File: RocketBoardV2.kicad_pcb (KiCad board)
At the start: 2 copper layers, 12 parts, among them IC1 W25Q256JVEIQ, J1 10118194-0001LF, J3 Conn_01x03_Pin, U1 SC0914_13_, U2 W25Q16JVUXIQ_TR, U3 BMI270, U4 TPS62420DRCR, Y1 ABM8-272-T3

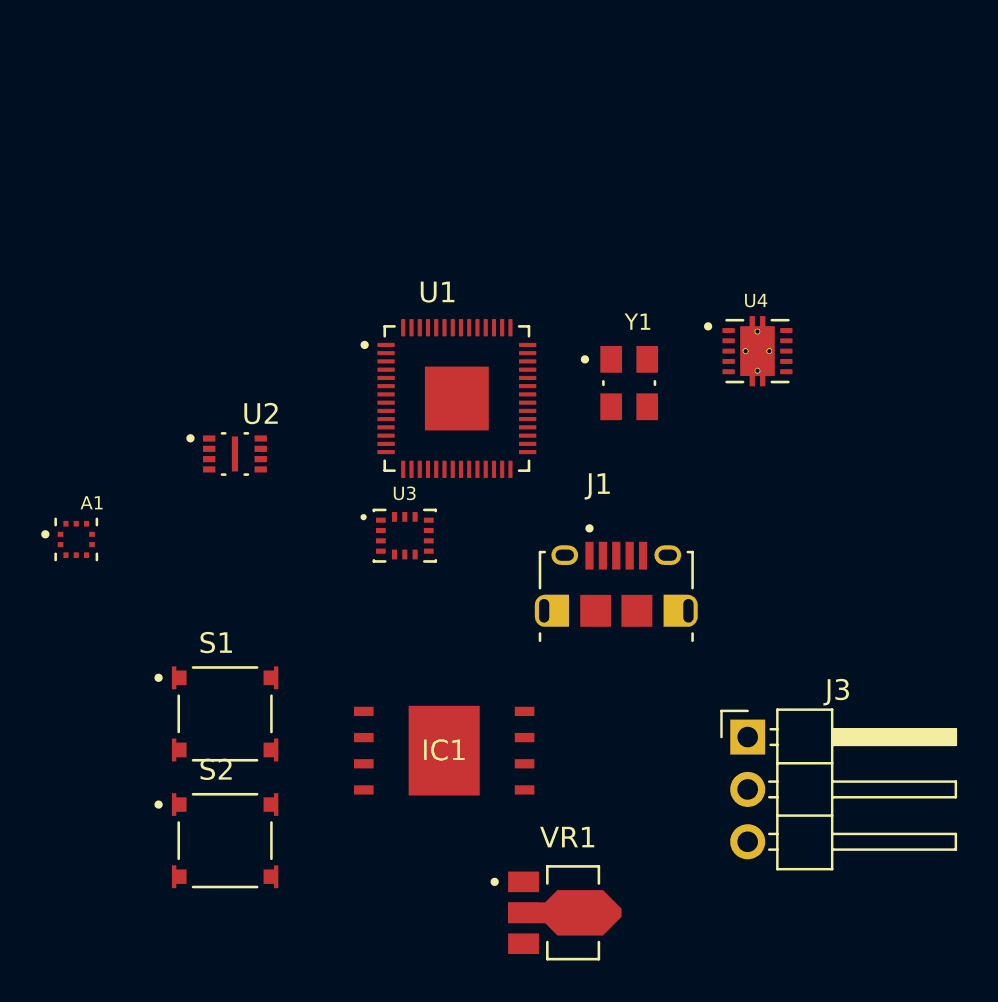
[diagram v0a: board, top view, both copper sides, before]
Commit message: basic layout
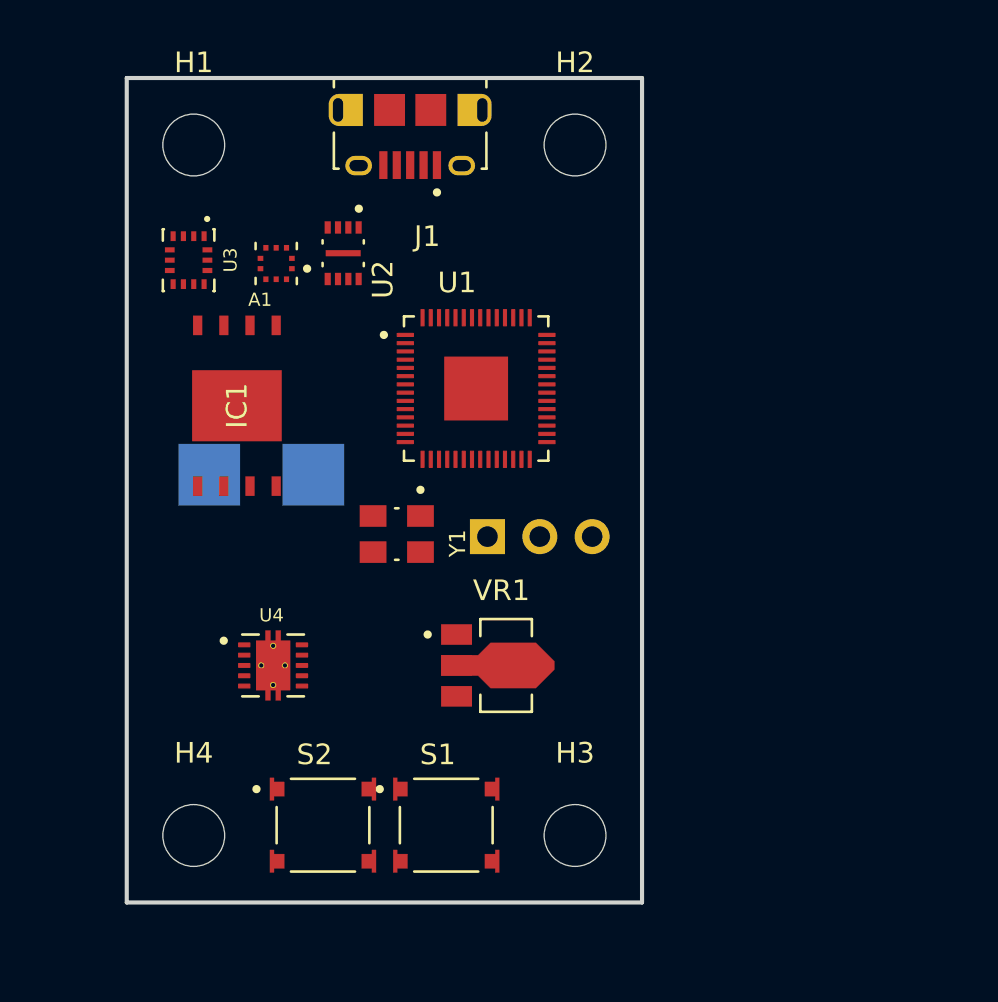
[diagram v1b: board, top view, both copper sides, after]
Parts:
- added H1: MountingHole, MountingHole:MountingHole_3mm, F.Cu at (125.5, 69.0)
- added H2: MountingHole, MountingHole:MountingHole_3mm, F.Cu at (144.0, 69.0)
- added H3: MountingHole, MountingHole:MountingHole_3mm, F.Cu at (144.0, 102.5)
- added H4: MountingHole, MountingHole:MountingHole_3mm, F.Cu at (125.5, 102.5)
- added TP3: TestPoint, TestPoint:TestPoint_Pad_3.0x3.0mm, B.Cu at (126.2, 85.0)
- added TP4: TestPoint, TestPoint:TestPoint_Pad_3.0x3.0mm, B.Cu at (131.3, 85.0)
- J3: moved to B.Cu
- moved U4 28.0 mm to (129.3, 94.2)
- moved J1 26.3 mm to (136.0, 67.3), turned to 180 degrees
- moved IC1 19.5 mm to (127.6, 81.7), turned to 90 degrees
- moved U3 17.0 mm to (125.2, 74.6), turned to -90 degrees
- moved A1 16.5 mm to (129.5, 74.8), turned to 180 degrees
- moved J3 15.9 mm to (139.8, 88.0), turned to -90 degrees
- moved Y1 13.4 mm to (135.3, 87.9), turned to -90 degrees
- moved VR1 12.4 mm to (140.2, 94.2)
- moved S1 12.0 mm to (137.8, 102.0)
- moved U2 11.1 mm to (132.8, 74.2), turned to -90 degrees
- moved S2 4.81 mm to (131.8, 102.0)
- moved U1 1.05 mm to (139.2, 80.8)
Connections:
- net VBUS renamed Net-(D4-A)
- IC1 pad 3: +3V3 -> Net-(IC1-DO_(IO1)_2)
- IC1 pad 7: +3V3 -> Net-(IC1-IO3)
- J3 pad 1: unconnected-(J3-Pin_1-Pad1) -> /SERVO
- U1 pad 7: unconnected-(U1-GPIO5-Pad7) -> /SERVO
- VR1 pad 1: unconnected-(VR1-OUTPUT-Pad1) -> Net-(D3-A)
- VR1 pad 2: unconnected-(VR1-COMMON-Pad2) -> GND
- VR1 pad 3: unconnected-(VR1-INPUT-Pad3) -> +BATT
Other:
- board outline added: 25 x 40 mm
